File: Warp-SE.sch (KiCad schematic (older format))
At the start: 9 parts

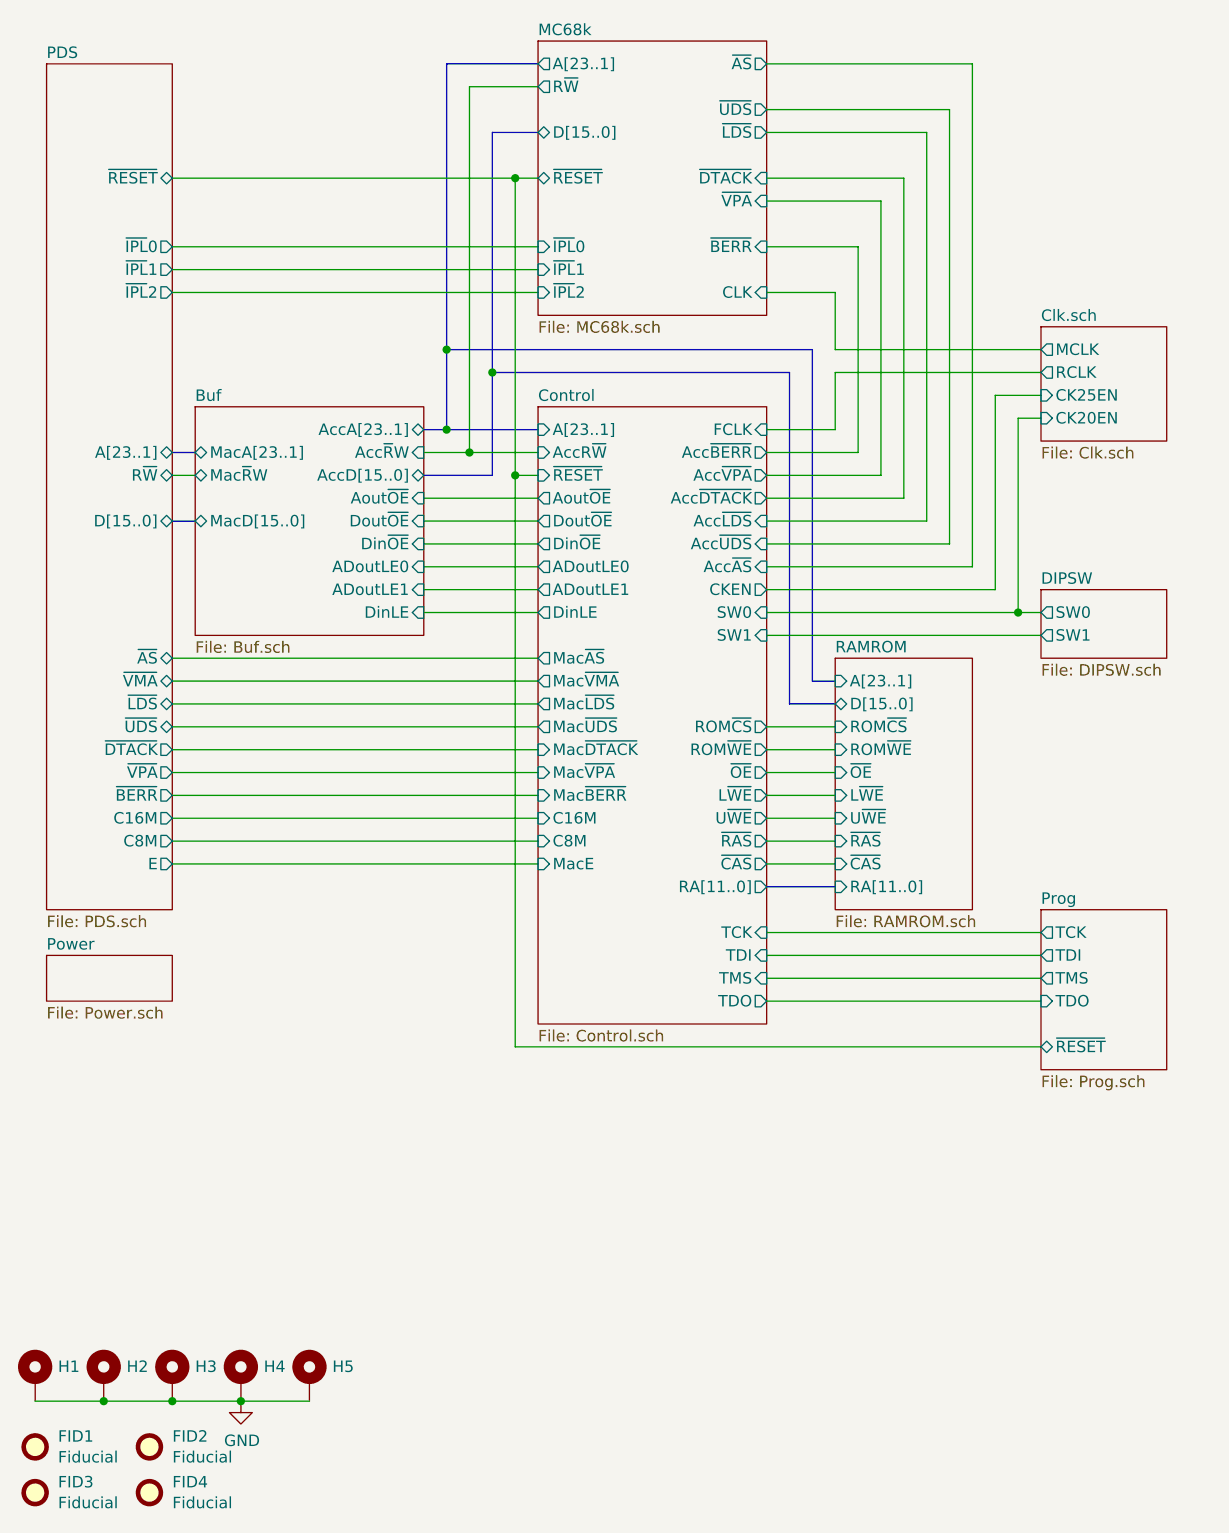
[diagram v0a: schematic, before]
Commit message: Moving toward new update system
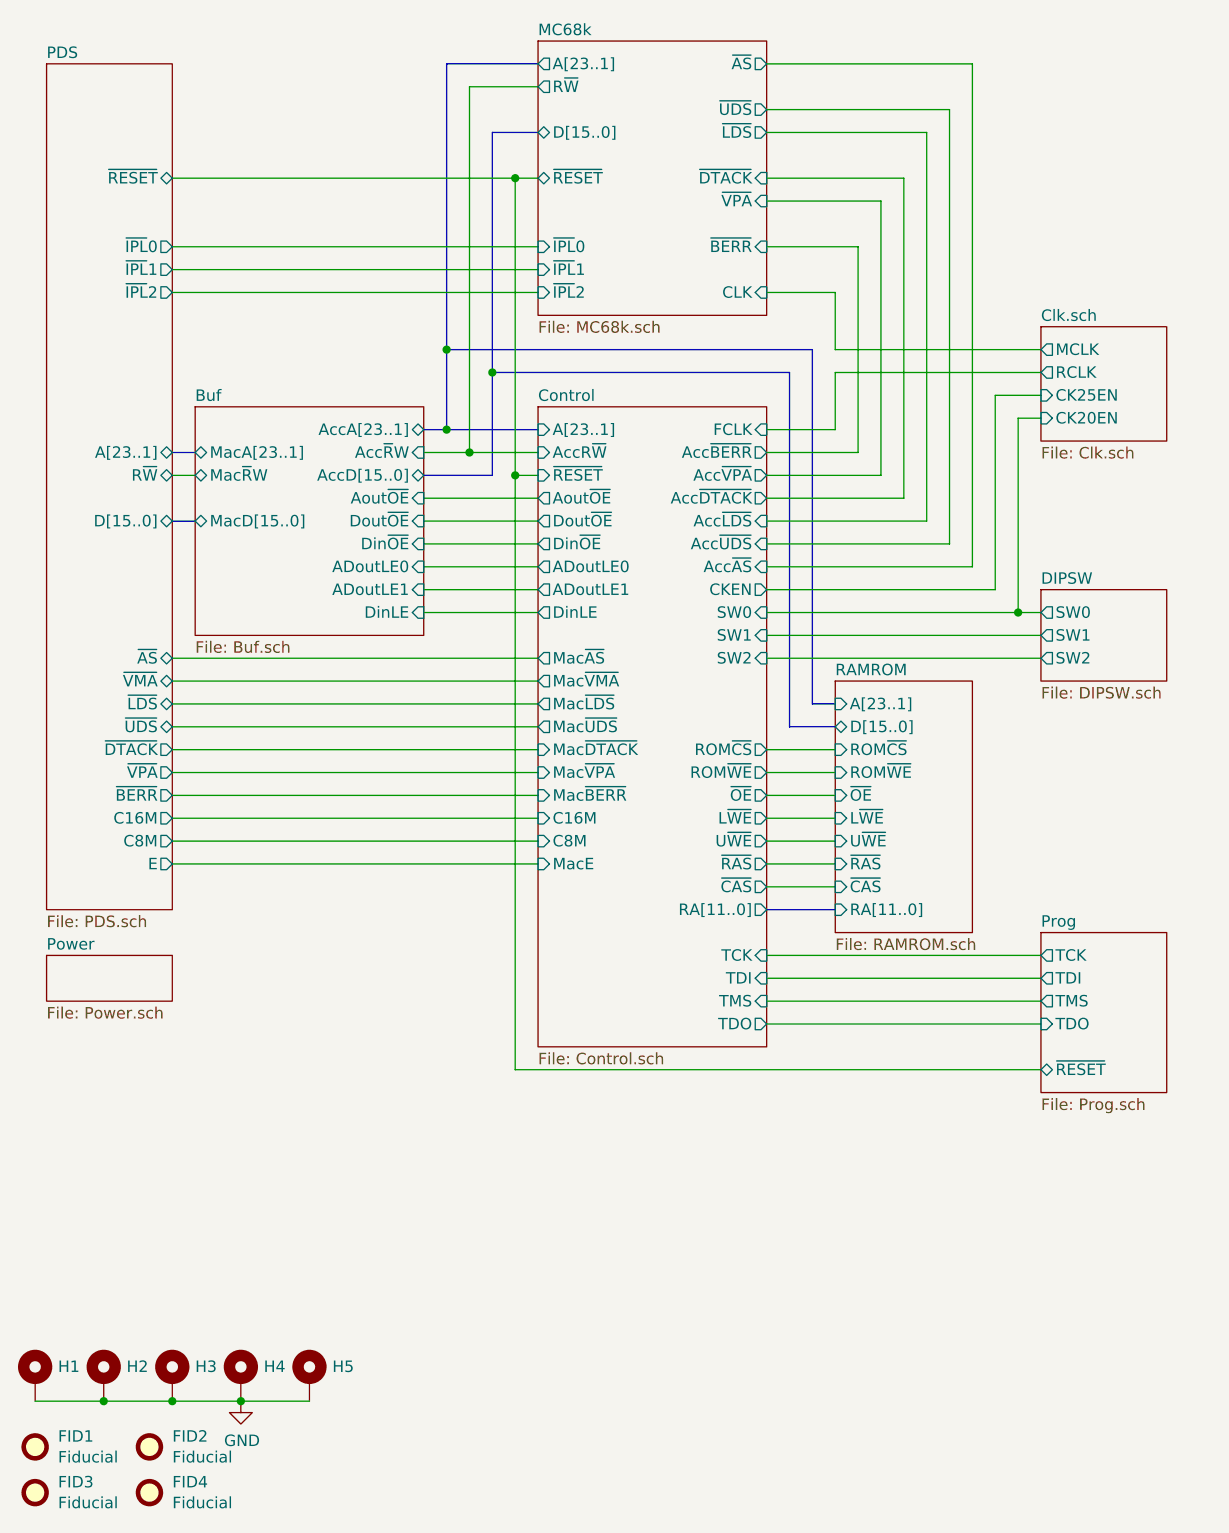
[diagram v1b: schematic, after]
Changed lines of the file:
@@
 F13 "ADoutLE1" I R 2700 3400 50
 $EndSheet
-Wire Bus Line
-	4300 2450 4300 3900
 Wire Wire Line
 	2900 1200 2900 2800
@@
 F15 "CLK" I R 4200 2100 50
 $EndSheet
-Wire Bus Line
-	4400 2350 4400 3800
 Connection ~ 2800 2350
 Wire Bus Line
@@
 	4500 2100 4500 2350
 $Sheet
-S 5400 3400 550  300
+S 5400 3400 550  400
 U 61A87B62
 F0 "DIPSW" 50
@@
 F2 "SW0" O L 5400 3500 50
 F3 "SW1" O L 5400 3600 50
+F4 "SW2" O L 5400 3700 50
 $EndSheet
 Wire Wire Line
@@
 	5400 3600 4200 3600
 $Sheet
-S 3200 2600 1000 2700
+S 3200 2600 1000 2800
 U 5F723173
 F0 "Control" 50
@@
 F15 "Acc~LDS~" I R 4200 3100 50
 F16 "Acc~AS~" I R 4200 3300 50
-F17 "~OE~" O R 4200 4200 50
+F17 "~OE~" O R 4200 4300 50
 F18 "Mac~UDS~" O L 3200 4000 50
 F19 "Mac~LDS~" O L 3200 3900 50
 F20 "Acc~VPA~" O R 4200 2900 50
 F21 "AccR~W~" I L 3200 2800 50
-F22 "L~WE~" O R 4200 4300 50
-F23 "U~WE~" O R 4200 4400 50
-F24 "~RAS~" O R 4200 4500 50
-F25 "~CAS~" O R 4200 4600 50
-F26 "ROM~CS~" O R 4200 4000 50
+F22 "L~WE~" O R 4200 4400 50
+F23 "U~WE~" O R 4200 4500 50
+F24 "~RAS~" O R 4200 4600 50
+F25 "~CAS~" O R 4200 4700 50
+F26 "ROM~CS~" O R 4200 4100 50
 F27 "DinLE" O L 3200 3500 50
 F28 "Dout~OE~" O L 3200 3100 50
 F29 "Aout~OE~" O L 3200 3000 50
 F30 "Din~OE~" O L 3200 3200 50
-F31 "RA[11..0]" O R 4200 4700 50
+F31 "RA[11..0]" O R 4200 4800 50
 F32 "A[23..1]" I L 3200 2700 50
 F33 "ADoutLE0" O L 3200 3300 50
 F34 "ADoutLE1" O L 3200 3400 50
-F35 "ROM~WE~" O R 4200 4100 50
+F35 "ROM~WE~" O R 4200 4200 50
 F36 "SW0" I R 4200 3500 50
 F37 "SW1" I R 4200 3600 50
 F38 "CKEN" O R 4200 3400 50
-F39 "TDI" I R 4200 5000 50
-F40 "TMS" I R 4200 5100 50
-F41 "TCK" I R 4200 4900 50
-F42 "TDO" O R 4200 5200 50
+F39 "TDI" I R 4200 5100 50
+F40 "TMS" I R 4200 5200 50
+F41 "TCK" I R 4200 5000 50
+F42 "TDO" O R 4200 5300 50
+F43 "SW2" I R 4200 3700 50
 $EndSheet
 Wire Wire Line
@@
 $EndSheet
 $Sheet
-S 5400 4800 550  700
+S 5400 4900 550  700
 U 61AA52C4
 F0 "Prog" 50
 F1 "Prog.sch" 50
-F2 "TCK" O L 5400 4900 50
-F3 "TDI" O L 5400 5000 50
-F4 "TMS" O L 5400 5100 50
-F5 "TDO" I L 5400 5200 50
-F6 "~RESET~" T L 5400 5400 50
-$EndSheet
+F2 "TCK" O L 5400 5000 50
+F3 "TDI" O L 5400 5100 50
+F4 "TMS" O L 5400 5200 50
+F5 "TDO" I L 5400 5300 50
+F6 "~RESET~" T L 5400 5500 50
+$EndSheet
+Wire Wire Line
+	4200 4200 4500 4200
+Wire Bus Line
+	4400 3900 4500 3900
 Wire Wire Line
 	4200 4100 4500 4100
-Wire Bus Line
-	4400 3800 4500 3800
-Wire Wire Line
-	4200 4000 4500 4000
+Wire Wire Line
+	4200 4500 4500 4500
 Wire Wire Line
 	4200 4400 4500 4400
+Wire Bus Line
+	4200 4800 4500 4800
 Wire Wire Line
 	4200 4300 4500 4300
-Wire Bus Line
+Wire Wire Line
 	4200 4700 4500 4700
-Wire Wire Line
-	4200 4200 4500 4200
+Wire Bus Line
+	4500 4000 4300 4000
 Wire Wire Line
 	4200 4600 4500 4600
-Wire Bus Line
-	4500 3900 4300 3900
-Wire Wire Line
-	4200 4500 4500 4500
-$Sheet
-S 4500 3700 600  1100
+$Sheet
+S 4500 3800 600  1100
 U 5F723900
 F0 "RAMROM" 50
 F1 "RAMROM.sch" 50
-F2 "~RAS~" I L 4500 4500 50
-F3 "D[15..0]" B L 4500 3900 50
-F4 "~CAS~" I L 4500 4600 50
-F5 "~OE~" I L 4500 4200 50
-F6 "RA[11..0]" I L 4500 4700 50
-F7 "L~WE~" I L 4500 4300 50
-F8 "U~WE~" I L 4500 4400 50
-F9 "ROM~CS~" I L 4500 4000 50
-F10 "A[23..1]" I L 4500 3800 50
-F11 "ROM~WE~" I L 4500 4100 50
-$EndSheet
+F2 "~RAS~" I L 4500 4600 50
+F3 "D[15..0]" B L 4500 4000 50
+F4 "~CAS~" I L 4500 4700 50
+F5 "~OE~" I L 4500 4300 50
+F6 "RA[11..0]" I L 4500 4800 50
+F7 "L~WE~" I L 4500 4400 50
+F8 "U~WE~" I L 4500 4500 50
+F9 "ROM~CS~" I L 4500 4100 50
+F10 "A[23..1]" I L 4500 3900 50
+F11 "ROM~WE~" I L 4500 4200 50
+$EndSheet
+Wire Wire Line
+	4200 5100 5400 5100
+Wire Wire Line
+	4200 5300 5400 5300
+Wire Wire Line
+	4200 5200 5400 5200
 Wire Wire Line
 	4200 5000 5400 5000
 Wire Wire Line
-	4200 5200 5400 5200
-Wire Wire Line
-	4200 5100 5400 5100
-Wire Wire Line
-	4200 4900 5400 4900
-Wire Wire Line
-	3100 2900 3100 5400
-Wire Wire Line
-	3100 5400 5400 5400
+	3100 2900 3100 5500
+Wire Wire Line
+	3100 5500 5400 5500
 Connection ~ 3100 2900
+Wire Wire Line
+	4200 3700 5400 3700
+Wire Bus Line
+	4300 2450 4300 4000
+Wire Bus Line
+	4400 2350 4400 3900
 $EndSCHEMATC
